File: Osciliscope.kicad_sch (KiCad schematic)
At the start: 60 parts, among them J1 U.FL, J2 Conn_01x04_Socket, J3 U.FL, J4 Conn_01x04_Socket, J5 USB_C_Receptacle_USB2.0_14P, J6 Conn_01x02_MountingPin, SW1 RotaryEncoder_Switch, SW2 SW_SPST, SW3 SW_Nidec_CAS-120A1, SW4 SW_Nidec_CAS-120A1, SW5 RotaryEncoder_Switch, SW6 RotaryEncoder_Switch, U1 MCP1700x-330xxMB, U2 ADC082S101, U3 IP2721, U4 AZ1084-5.0, U5 TLV9061xDBV, U7 TLV9061xDBV, U8 MCP4251-104E/ML-ND

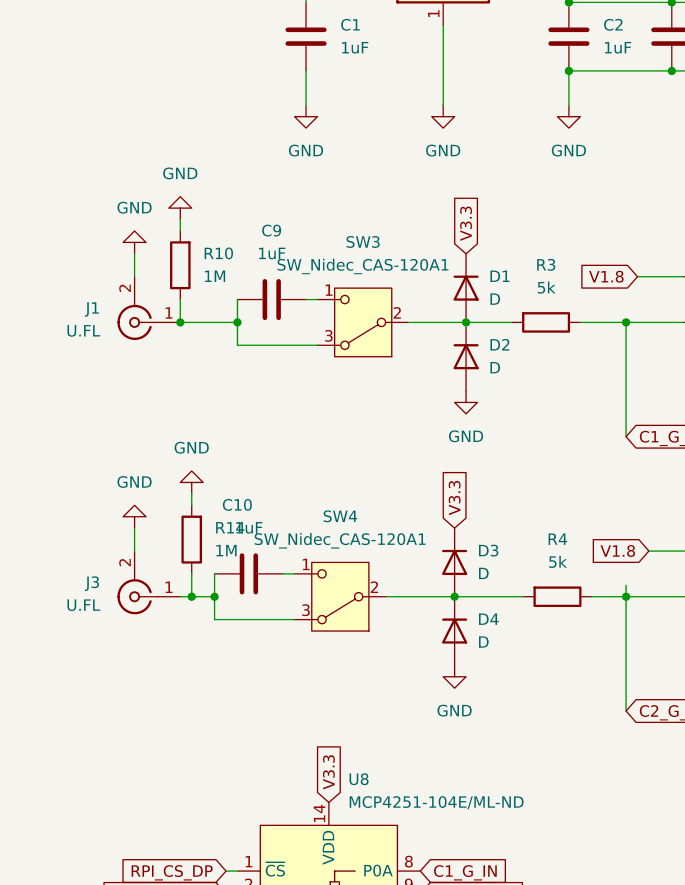
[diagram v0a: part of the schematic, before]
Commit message: Balls
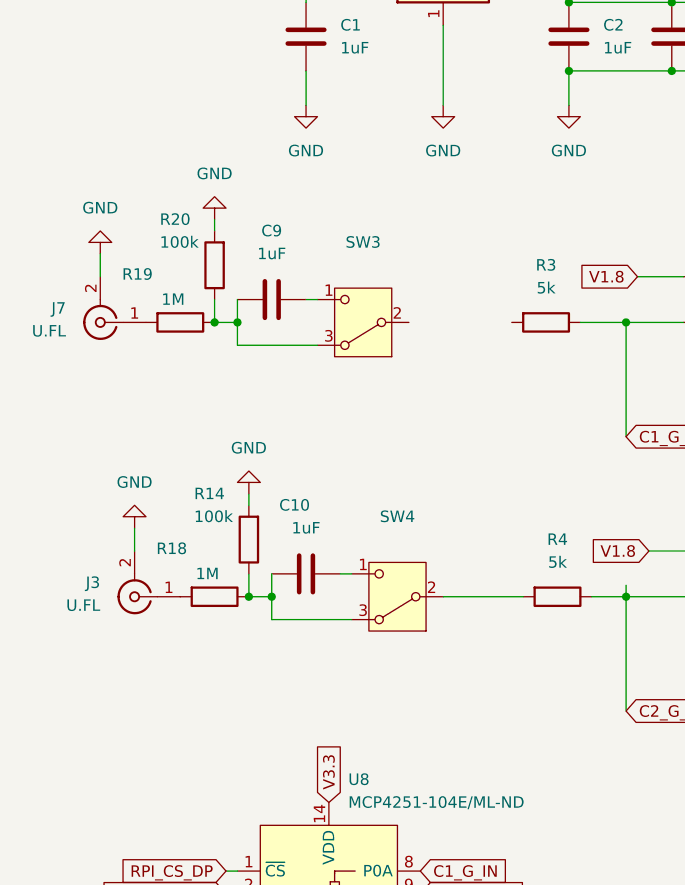
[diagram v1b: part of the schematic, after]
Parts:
- removed D1, D2, D3, D4: D, Diode_SMD:D_0201_0603Metric, symbol Device:D
- removed J1: U.FL, Connector_Coaxial:BNC_Amphenol_031-5539_Vertical, symbol PCM_JLCPCB-Extended:RF, Connector, U.FL
- removed R10: 1M, Capacitor_SMD:C_0603_1608Metric, symbol Device:R
- added J7: U.FL, Connector_Coaxial:BNC_Amphenol_031-5539_Vertical, symbol PCM_JLCPCB-Extended:RF, Connector, U.FL
- added R18, R19: 1M, Capacitor_SMD:C_0603_1608Metric, symbol Device:R
- added R20: 100k, Capacitor_SMD:C_0603_1608Metric, symbol Device:R
- R14: value 1M -> 100k
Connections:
- net GND: now also J7.2 (Ext), R20.2
- net at C10.1, R14.1, SW4.3 (A): now also R18.1; no longer J3.1 (In)
- net at C9.1, SW3.3 (A): now also R19.1, R20.1
- net at R3.2: no longer SW3.2 (B)
- new net: J7.1 (In), R19.2
- new net: J3.1 (In), R18.2
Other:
- moved on the sheet: C10, R14, SW4
